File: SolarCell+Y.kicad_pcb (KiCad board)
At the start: 6 copper layers, 50 x 50 mm, 73 parts, among them J1 symbols_XF2M-1015-1A, J2 U.FL-R-SMT-1, Q1 IRLML2803, U1 TTB12G51-Balun, U2 NDS8434, U3 TSL2561, U4 Value

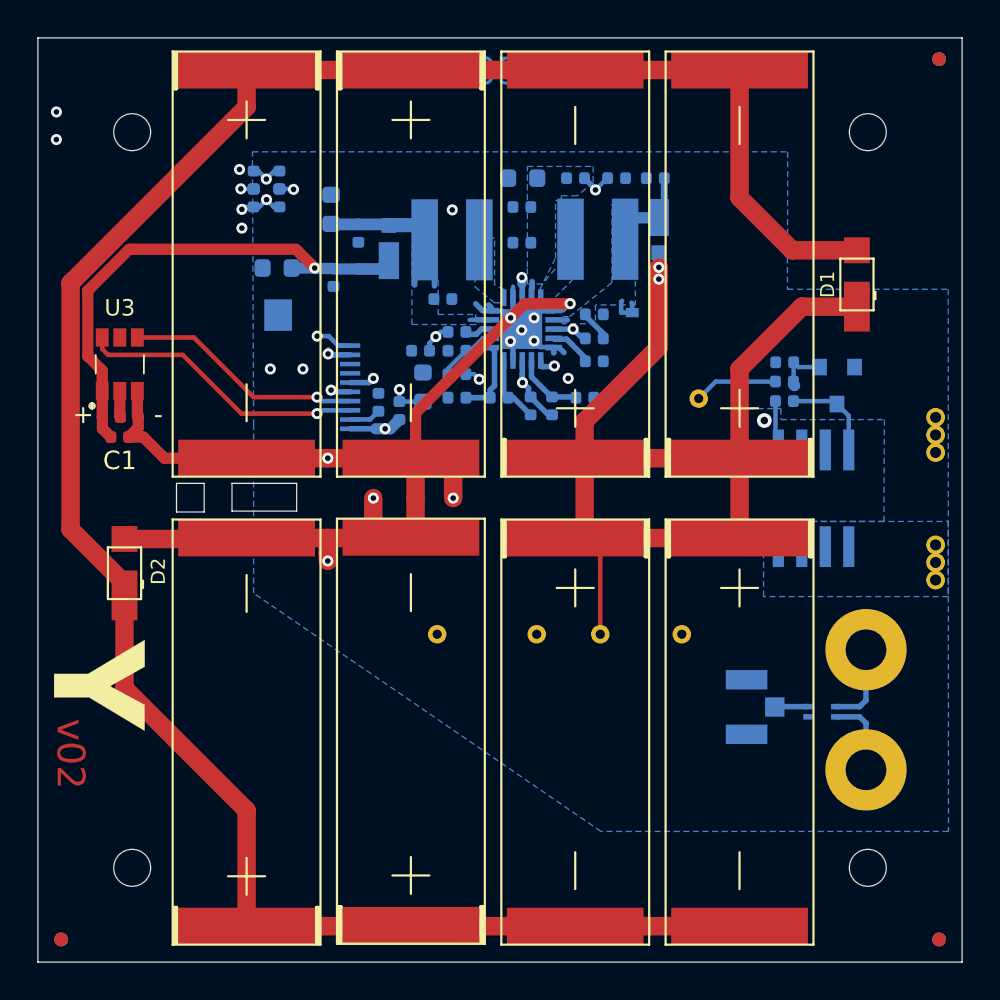
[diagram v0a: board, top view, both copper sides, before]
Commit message: Fixed magnetorquer coils
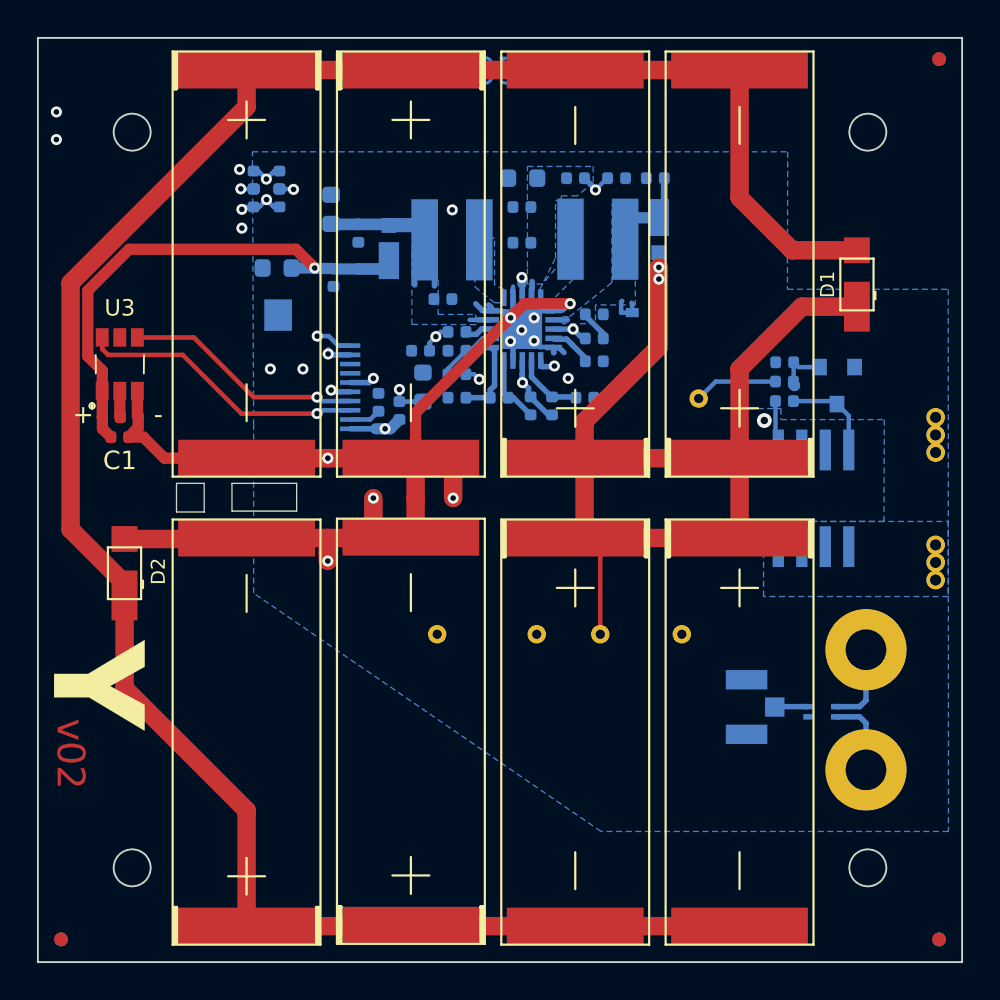
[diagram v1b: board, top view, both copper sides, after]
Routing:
- net /coil: track 13368.3 -> 13222.1 mm
